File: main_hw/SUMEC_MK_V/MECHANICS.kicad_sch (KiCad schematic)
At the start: 14 parts, among them SW2 SW_Push, SW3 SW_Push, SW4 SW_Push, SW5 SW_Push

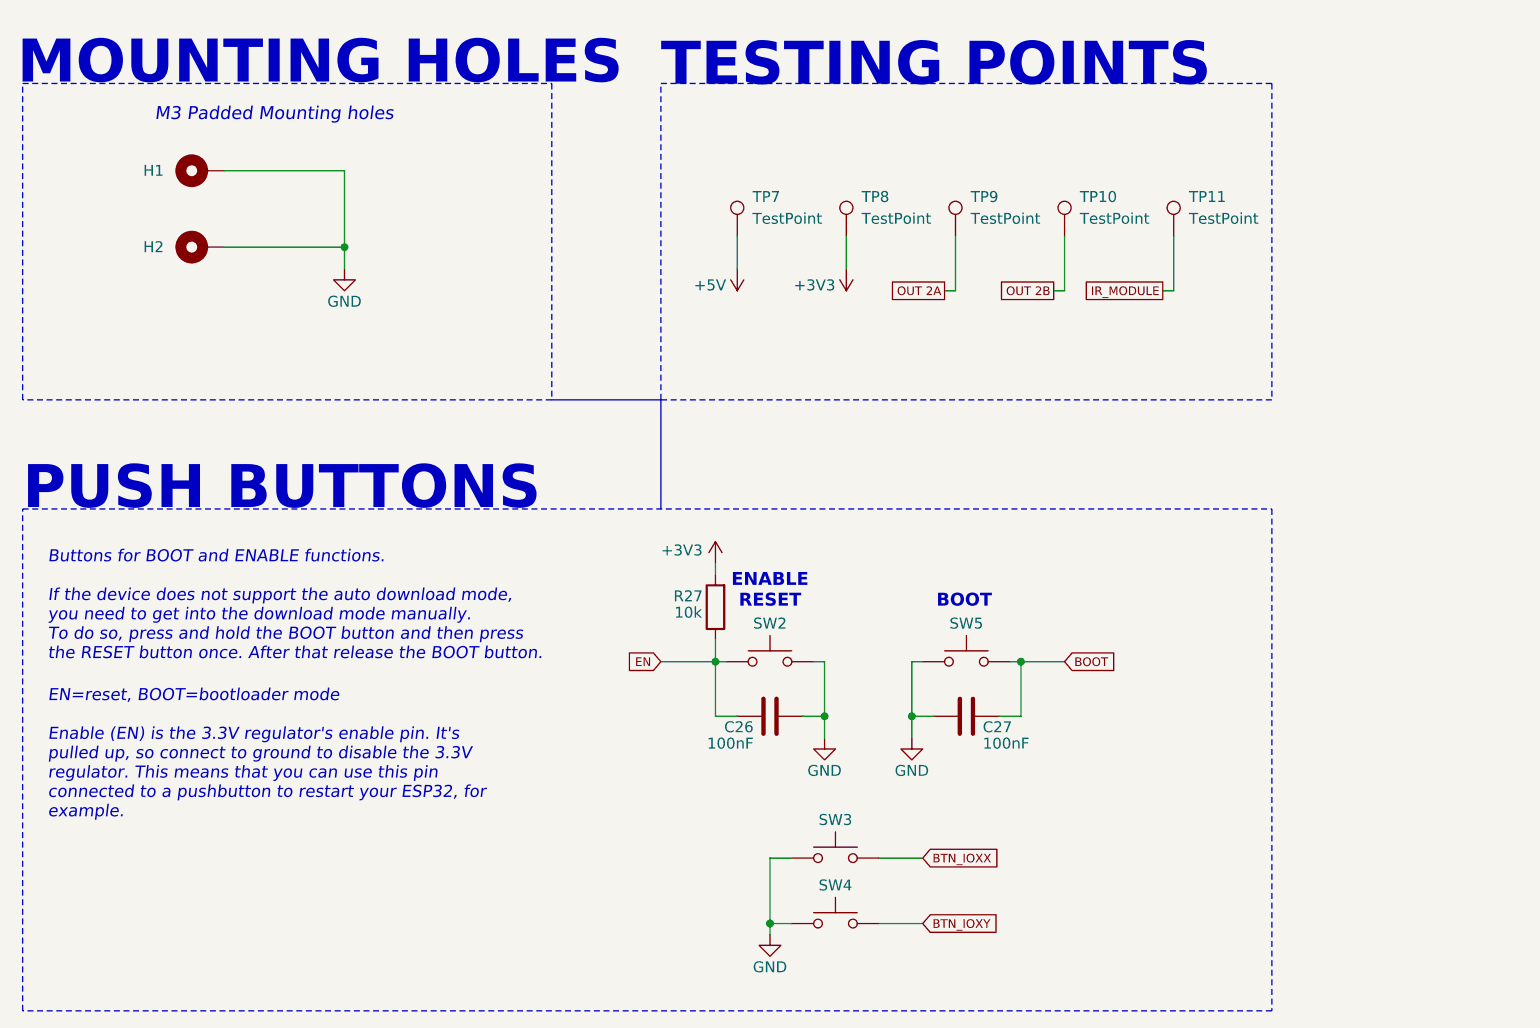
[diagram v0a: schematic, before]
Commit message: SUMEC MKIV
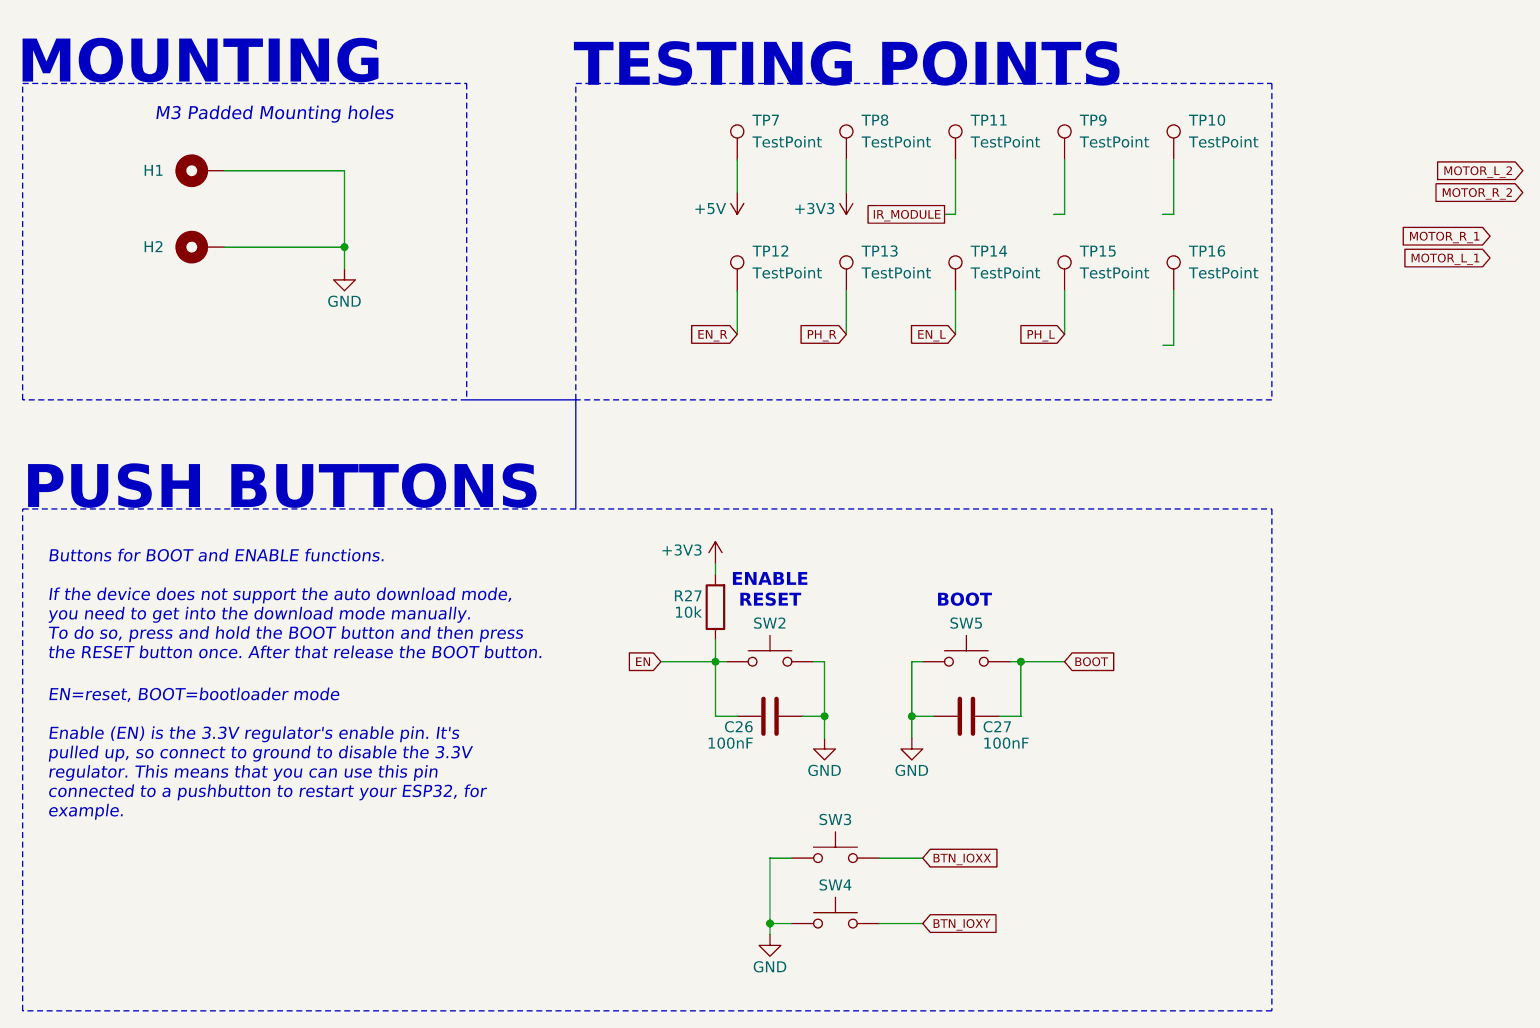
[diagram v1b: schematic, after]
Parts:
- added TP12, TP13, TP14, TP15, TP16: TestPoint, TestPoint:TestPoint_Pad_1.0x1.0mm, symbol Connector:TestPoint
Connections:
- net OUT 2A: no longer names the net of TP9.1
- net OUT 2B: no longer names the net of TP10.1
- new net EN_L: TP14.1
- new net EN_R: TP12.1
- new net PH_L: TP15.1
- new net PH_R: TP13.1
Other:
- note added: "MOUNTING"
- note removed: "MOUNTING HOLES"
- moved on the sheet: TP10, TP11, TP7, TP8, TP9
